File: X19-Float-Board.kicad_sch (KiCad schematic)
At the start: 5 parts

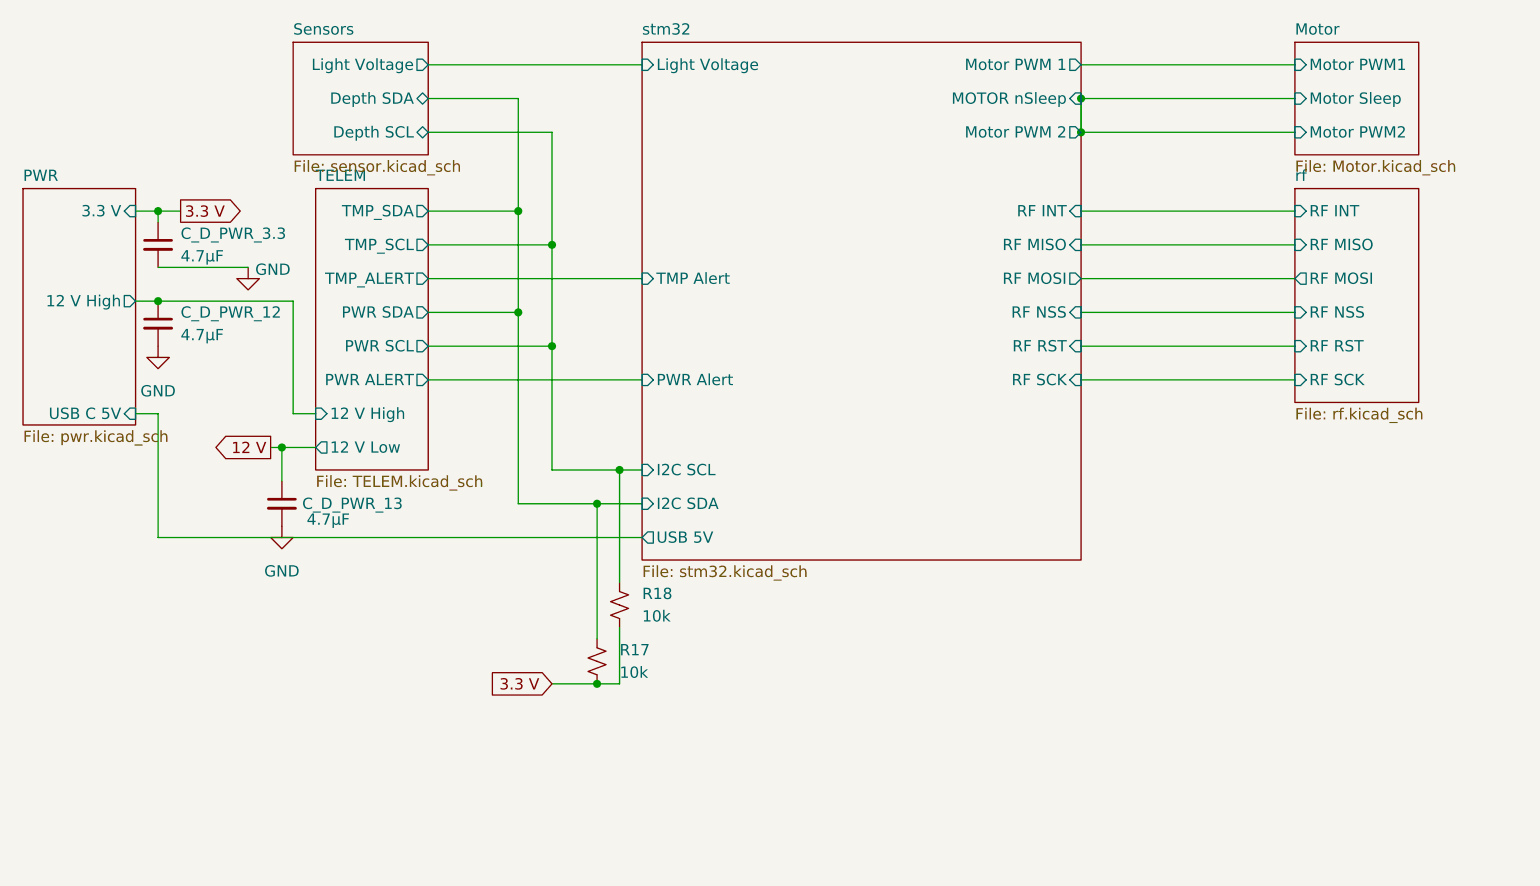
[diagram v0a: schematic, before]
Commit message: footprints
footprints
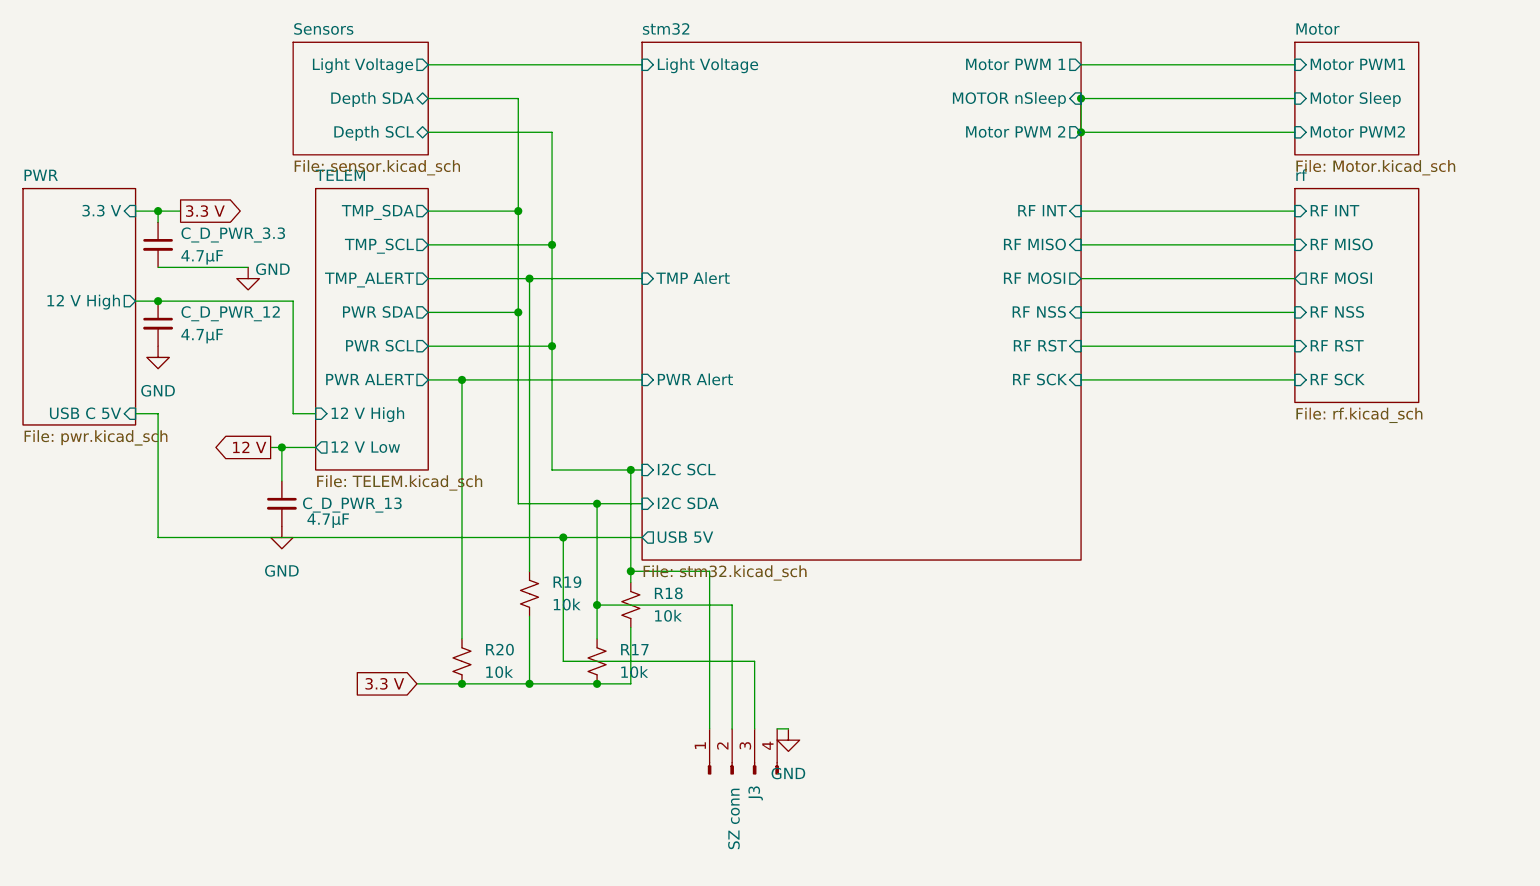
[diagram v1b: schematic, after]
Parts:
- added J3: SZ conn, symbol Connector:Conn_01x04_Pin
- added R19, R20: 10k, symbol Device:R_Small_US
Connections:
- net 3.3 V: now also R19.2, R20.2
- net GND: now also J3.4 (Pin_4)
- net PWR/USB C 5V: now also J3.3 (Pin_3)
- net Sensors/Depth SCL: now also J3.1 (Pin_1)
- net Sensors/Depth SDA: now also J3.2 (Pin_2)
- net TELEM/PWR ALERT: now also R20.1
- net TELEM/TMP_ALERT: now also R19.1
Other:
- moved on the sheet: R18
